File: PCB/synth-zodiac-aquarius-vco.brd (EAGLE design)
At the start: 76.1 x 72.4 mm, 59 parts, among them Q1 PMP4201, U1 TL074A, U2 LM393, U3 CD4066

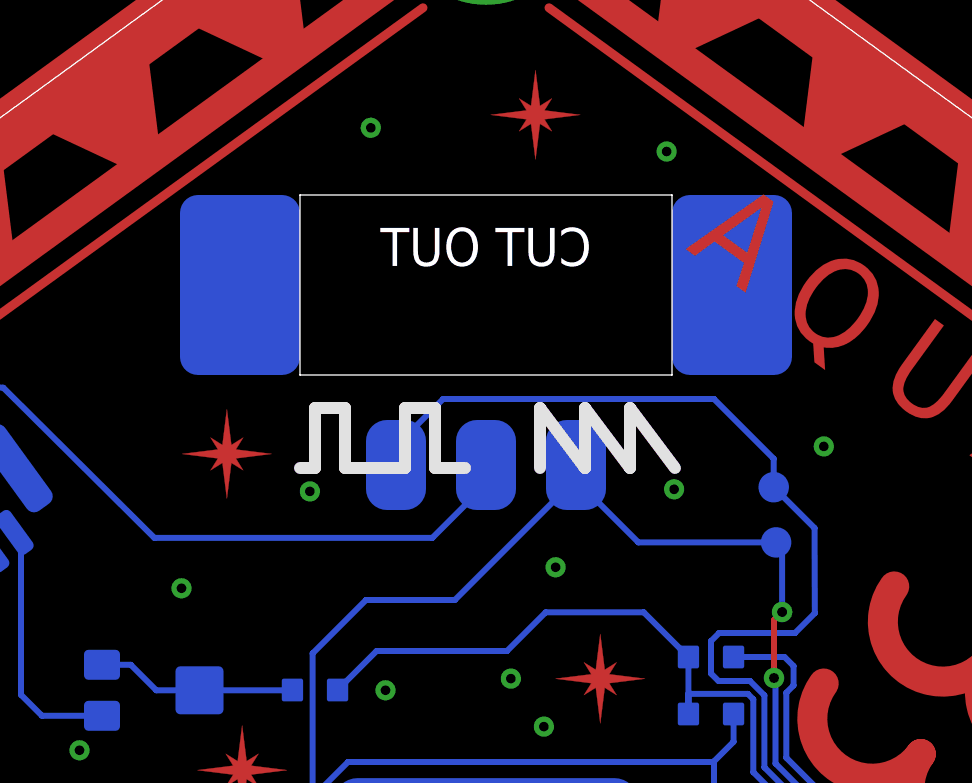
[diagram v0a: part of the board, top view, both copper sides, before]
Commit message: Perhaps final Rev. A?
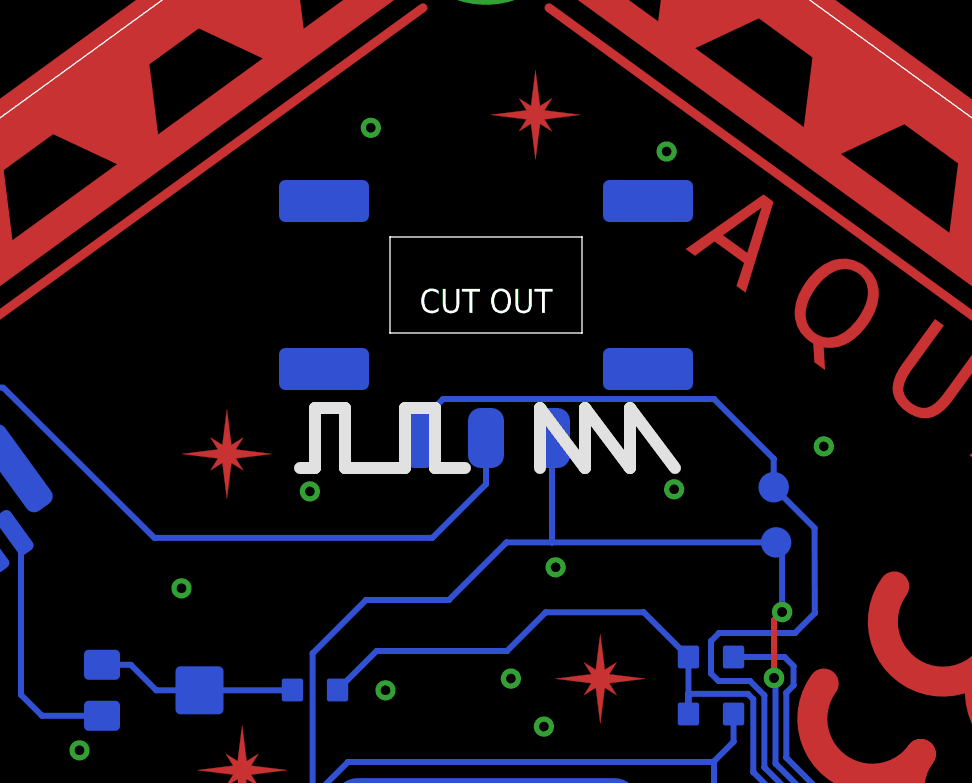
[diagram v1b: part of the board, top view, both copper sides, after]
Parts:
- MODE: device switch-thd:SS-12-F45-PNL-SMT -> switch-thd:SS-12-F45-PNL-SMT-2
- flipped MODE to the top
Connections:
- net GND: now also MODE.MTG3, MODE.MTG4
- net PULSE: now also MODE.A; no longer MODE.B
- net SAW: now also MODE.B; no longer MODE.A
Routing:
- net PULSE: track 57.2 -> 55.9 mm
- net VCO_OUT: track 48.9 -> 49.8 mm
- net SAW: track 89.9 -> 90.7 mm
